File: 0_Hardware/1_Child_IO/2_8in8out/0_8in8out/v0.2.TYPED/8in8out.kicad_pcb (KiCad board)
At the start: 2 copper layers, 100.1 x 86.4 mm, 56 parts, among them IC1 ATTINY48-A, J1 RJ45, J2 RJ45, J3 CONN_6, K110 T771D10, K120 T771D10, K130 T771D10, K140 T771D10, K150 T771D10, K160 T771D10, K170 T771D10, K180 T771D10, P1 CONN_5, P100 CONN_2, P101 CONN_2, P102 CONN_2, P103 CONN_2, P105 CONN_2, P106 CONN_2, P110 CONN_2, P120 CONN_2, P130 CONN_2, P140 CONN_2, P150 CONN_2, P160 CONN_2, P170 CONN_2, P180 CONN_2, P2 CONN_5, P3 CONN_10X2, U1 7805, U2 ULN2803, U3 LTV847, U4 LTV847

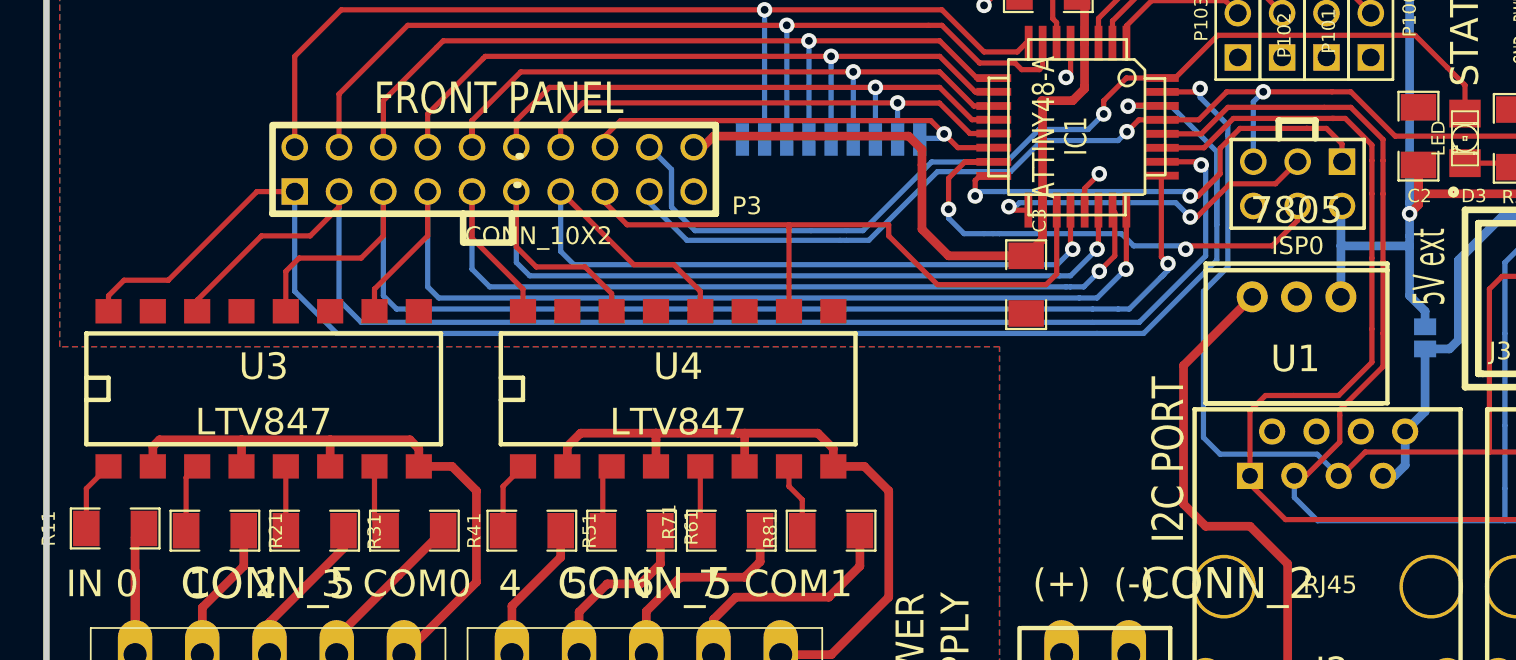
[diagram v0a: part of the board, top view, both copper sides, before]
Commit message: skilkscreen
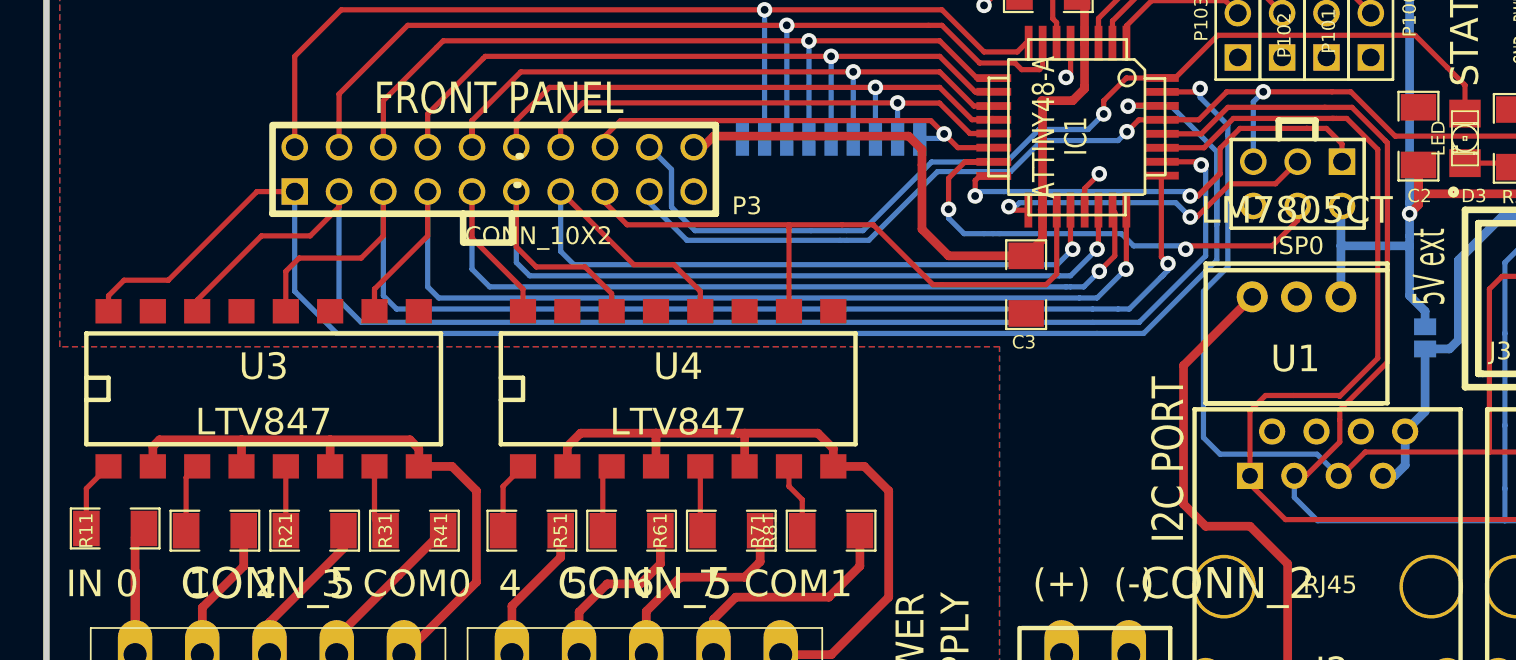
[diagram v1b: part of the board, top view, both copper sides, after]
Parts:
- U1: value 7805 -> LM7805CT
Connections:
- U1 pad 1: (no net) -> +12V
- U1 pad 2: (no net) -> GND
- U1 pad 3: (no net) -> +5V
